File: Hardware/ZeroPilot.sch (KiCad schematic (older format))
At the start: 2 parts

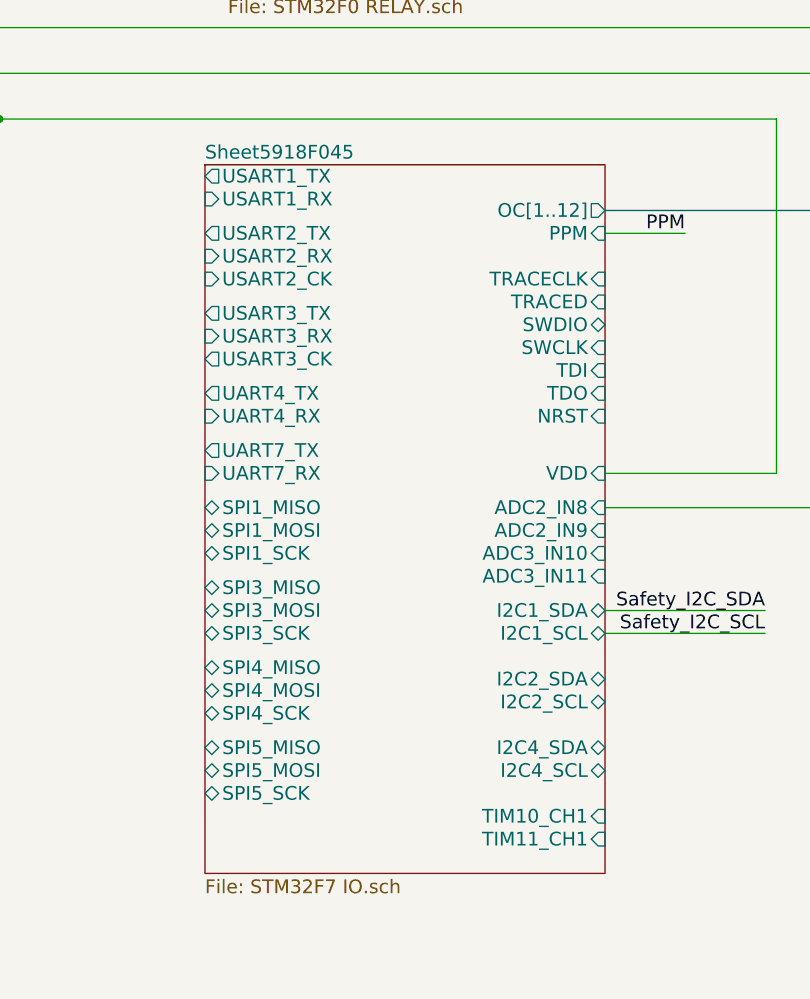
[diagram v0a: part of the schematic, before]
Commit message: Reconfiguring pinout round 2
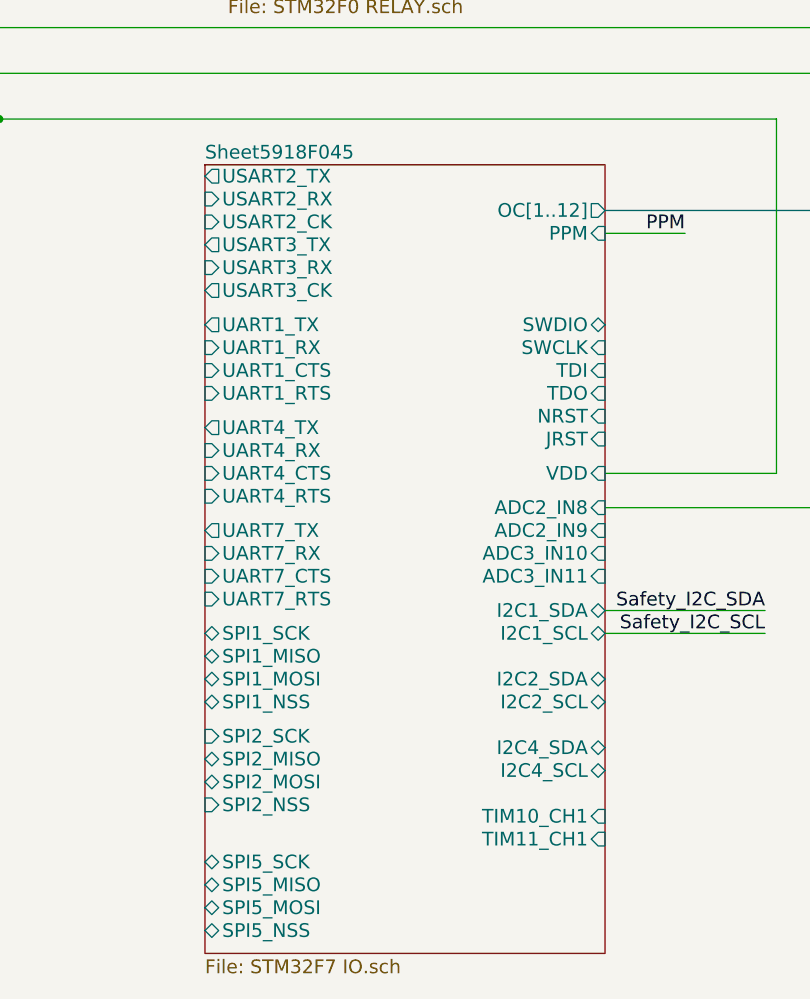
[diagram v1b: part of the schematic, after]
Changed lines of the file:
@@
-$EndSheet
-$Sheet
-S 4700 3100 1750 3100
-U 5918F046
-F0 "Sheet5918F045" 60
-F1 "STM32F7 IO.sch" 60
-F2 "PPM" I R 6450 3400 60
-F3 "OC[1..12]" O R 6450 3300 60
-F4 "TRACED" I R 6450 3700 60
-F5 "SWDIO" B R 6450 3800 60
-F6 "SWCLK" I R 6450 3900 60
-F7 "TDI" I R 6450 4000 60
-F8 "TDO" I R 6450 4100 60
-F9 "TRACECLK" I R 6450 3600 60
-F10 "NRST" I R 6450 4200 60
-F11 "I2C2_SDA" B R 6450 5350 60
-F12 "I2C2_SCL" B R 6450 5450 60
-F13 "SPI5_MISO" B L 4700 5650 60
-F14 "SPI5_MOSI" B L 4700 5750 60
-F15 "SPI5_SCK" B L 4700 5850 60
-F16 "USART2_TX" O L 4700 3400 60
-F17 "USART2_RX" I L 4700 3500 60
-F18 "SPI1_SCK" B L 4700 4800 60
-F19 "SPI1_MISO" B L 4700 4600 60
-F20 "SPI1_MOSI" B L 4700 4700 60
-F21 "I2C4_SCL" B R 6450 5750 60
-F22 "I2C4_SDA" B R 6450 5650 60
-F23 "UART7_TX" O L 4700 4350 60
-F24 "UART7_RX" I L 4700 4450 60
-F25 "SPI4_SCK" B L 4700 5500 60
-F26 "SPI4_MISO" B L 4700 5300 60
-F27 "SPI4_MOSI" B L 4700 5400 60
-F28 "USART1_RX" I L 4700 3250 60
-F29 "USART1_TX" O L 4700 3150 60
-F30 "USART3_TX" O L 4700 3750 60
-F31 "USART3_RX" I L 4700 3850 60
-F32 "USART3_CK" O L 4700 3950 60
-F33 "SPI3_SCK" B L 4700 5150 60
-F34 "SPI3_MISO" B L 4700 4950 60
-F35 "SPI3_MOSI" B L 4700 5050 60
-F36 "UART4_RX" I L 4700 4200 60
-F37 "UART4_TX" O L 4700 4100 60
-F38 "I2C1_SDA" B R 6450 5050 60
-F39 "I2C1_SCL" B R 6450 5150 60
-F40 "VDD" I R 6450 4450 60
-F41 "USART2_CK" I L 4700 3600 60
-F42 "ADC2_IN8" I R 6450 4600 60
-F43 "ADC2_IN9" I R 6450 4700 60
-F44 "ADC3_IN10" I R 6450 4800 60
-F45 "ADC3_IN11" I R 6450 4900 60
-F46 "TIM10_CH1" I R 6450 5950 60
-F47 "TIM11_CH1" I R 6450 6050 60
 $EndSheet
 $Sheet
@@
 F1 "HEADERS.sch" 60
 $EndSheet
+$Sheet
+S 4700 3100 1750 3450
+U 5918F046
+F0 "Sheet5918F045" 60
+F1 "STM32F7 IO.sch" 60
+F2 "PPM" I R 6450 3400 60
+F3 "OC[1..12]" O R 6450 3300 60
+F4 "SWDIO" B R 6450 3800 60
+F5 "SWCLK" I R 6450 3900 60
+F6 "TDI" I R 6450 4000 60
+F7 "TDO" I R 6450 4100 60
+F8 "NRST" I R 6450 4200 60
+F9 "I2C2_SDA" B R 6450 5350 60
+F10 "I2C2_SCL" B R 6450 5450 60
+F11 "I2C4_SCL" B R 6450 5750 60
+F12 "I2C4_SDA" B R 6450 5650 60
+F13 "I2C1_SDA" B R 6450 5050 60
+F14 "I2C1_SCL" B R 6450 5150 60
+F15 "VDD" I R 6450 4450 60
+F16 "ADC2_IN8" I R 6450 4600 60
+F17 "ADC2_IN9" I R 6450 4700 60
+F18 "ADC3_IN10" I R 6450 4800 60
+F19 "ADC3_IN11" I R 6450 4900 60
+F20 "TIM10_CH1" I R 6450 5950 60
+F21 "TIM11_CH1" I R 6450 6050 60
+F22 "SPI5_MISO" B L 4700 6250 60
+F23 "SPI5_MOSI" B L 4700 6350 60
+F24 "SPI5_SCK" B L 4700 6150 60
+F25 "USART2_TX" O L 4700 3150 60
+F26 "USART2_RX" I L 4700 3250 60
+F27 "SPI1_SCK" B L 4700 5150 60
+F28 "SPI1_MISO" B L 4700 5250 60
+F29 "SPI1_MOSI" B L 4700 5350 60
+F30 "UART7_TX" O L 4700 4700 60
+F31 "UART7_RX" I L 4700 4800 60
+F32 "UART1_RX" I L 4700 3900 60
+F33 "UART1_TX" O L 4700 3800 60
+F34 "USART3_TX" O L 4700 3450 60
+F35 "USART3_RX" I L 4700 3550 60
+F36 "USART3_CK" O L 4700 3650 60
+F37 "UART4_RX" I L 4700 4350 60
+F38 "UART4_TX" O L 4700 4250 60
+F39 "USART2_CK" I L 4700 3350 60
+F40 "SPI5_NSS" B L 4700 6450 60
+F41 "SPI2_MISO" B L 4700 5700 60
+F42 "SPI2_MOSI" B L 4700 5800 60
+F43 "UART4_CTS" I L 4700 4450 60
+F44 "UART7_CTS" I L 4700 4900 60
+F45 "UART7_RTS" I L 4700 5000 60
+F46 "SPI2_SCK" I L 4700 5600 60
+F47 "SPI2_NSS" I L 4700 5900 60
+F48 "UART4_RTS" I L 4700 4550 60
+F49 "UART1_CTS" I L 4700 4000 60
+F50 "UART1_RTS" I L 4700 4100 60
+F51 "SPI1_NSS" B L 4700 5450 60
+F52 "JRST" I R 6450 4300 60
+$EndSheet
 $EndSCHEMATC

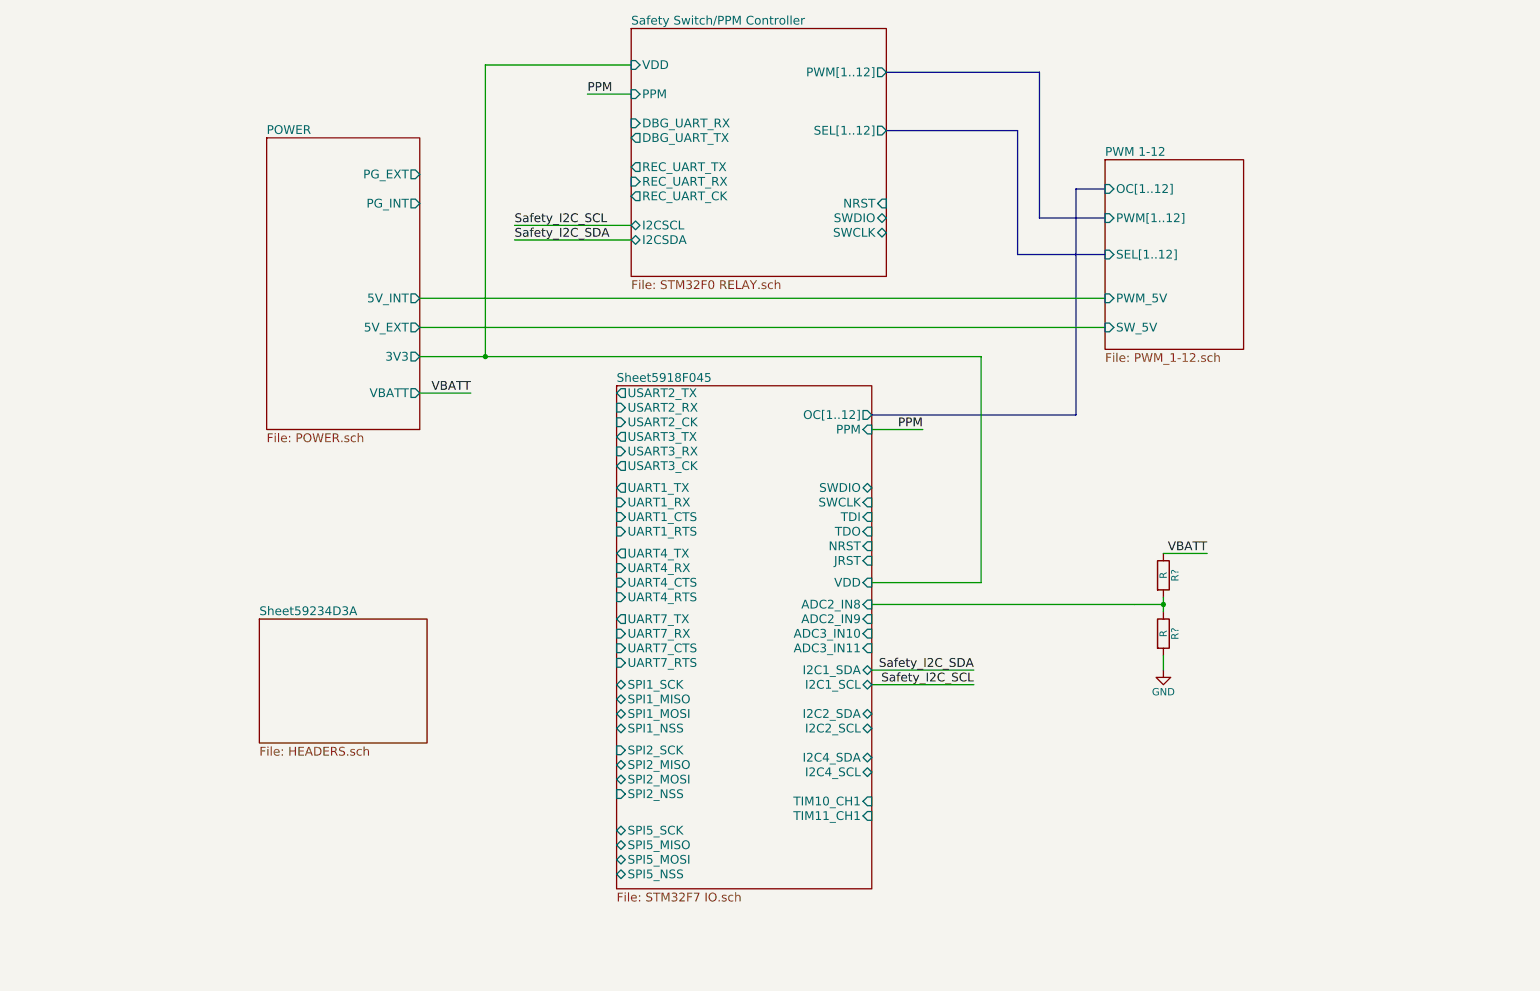
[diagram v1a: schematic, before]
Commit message: first rough draft without headers
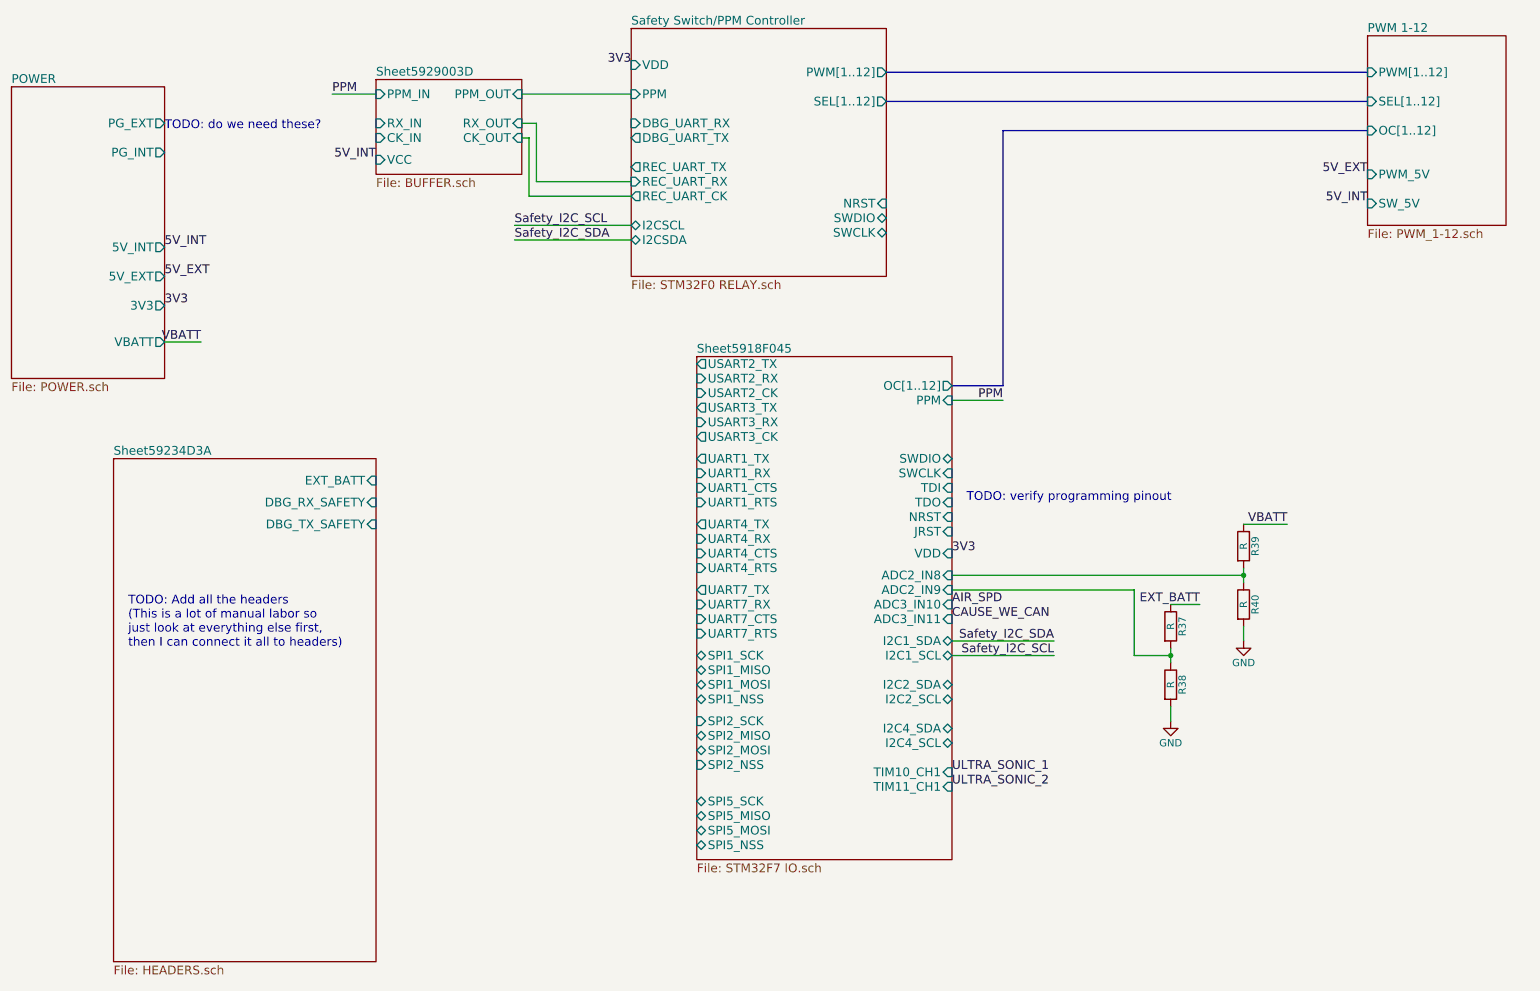
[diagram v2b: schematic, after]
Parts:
- added R37, R38: R, symbol R
- gave numbers to parts that had none: 2
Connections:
- net GND: now also R38.2
- net Sheet5918F045/ADC2_IN9: now also R37.2, R38.1
- new net EXT_BATT: R37.1
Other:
- note added: "TODO: Add all the headers\n(This is a lot of manual labor so \njust look at everything else first, \nthen I can connect it all to headers)\n"
- note added: "TODO: do we need these?\n"
- note added: "TODO: verify programming pinout"
- moved on the sheet: R39, R40
